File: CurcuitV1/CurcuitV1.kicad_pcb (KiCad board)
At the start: 2 copper layers, 40 x 40 mm, 46 parts, among them IC1 AS5600-ASOT, J1 Conn_01x07, J2 Conn_01x03, J3 Conn_01x02, J4 Conn_01x02, Q1 Q_NMOS_DGS, Q2 Q_NMOS_DGS, Q3 Q_NMOS_DGS, Q4 Q_NMOS_DGS, Q5 Q_NMOS_DGS, Q6 Q_NMOS_DGS, SW1 SW_Push, U1 IR2302, U2 IR2302, U3 IR2302, U4 STM32F303K8Tx, U5 LM1117MP-3.3, Y2 CSTNE16M0V530000R0

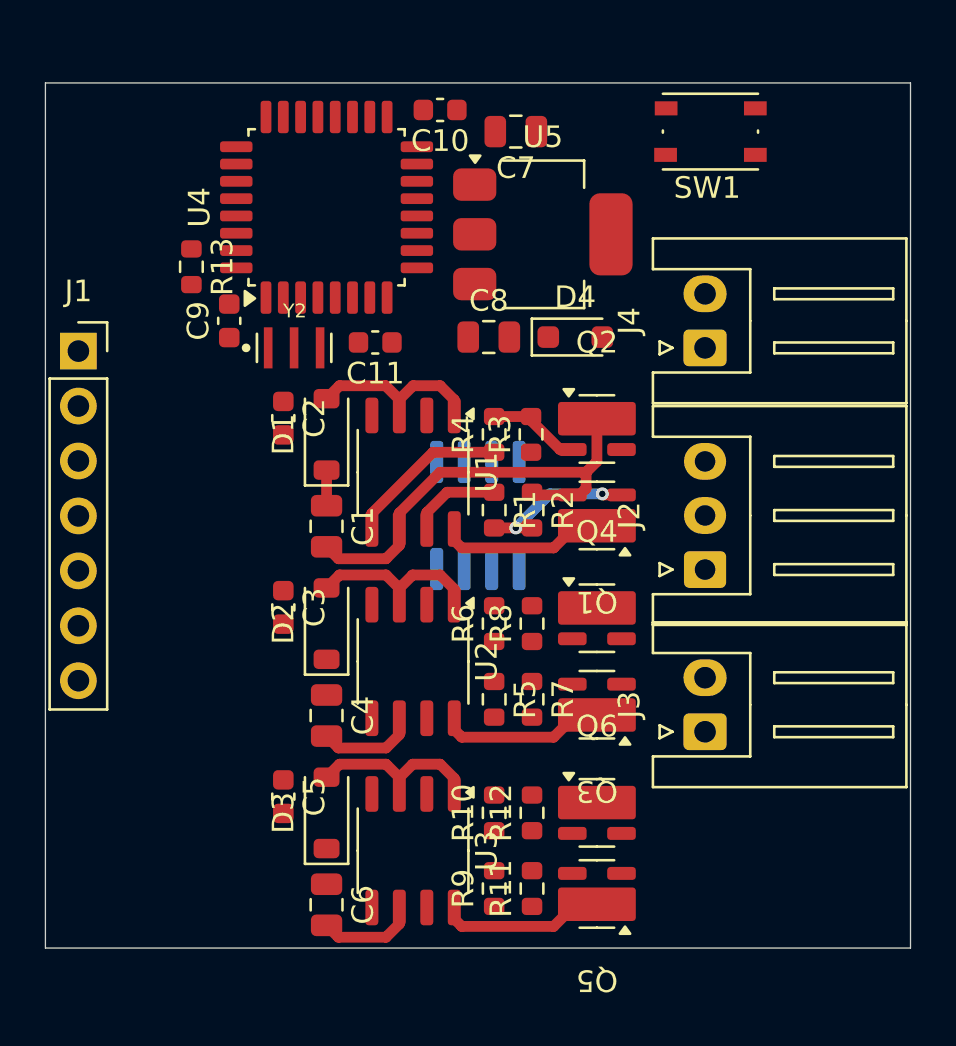
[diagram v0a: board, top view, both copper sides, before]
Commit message: 大体完成
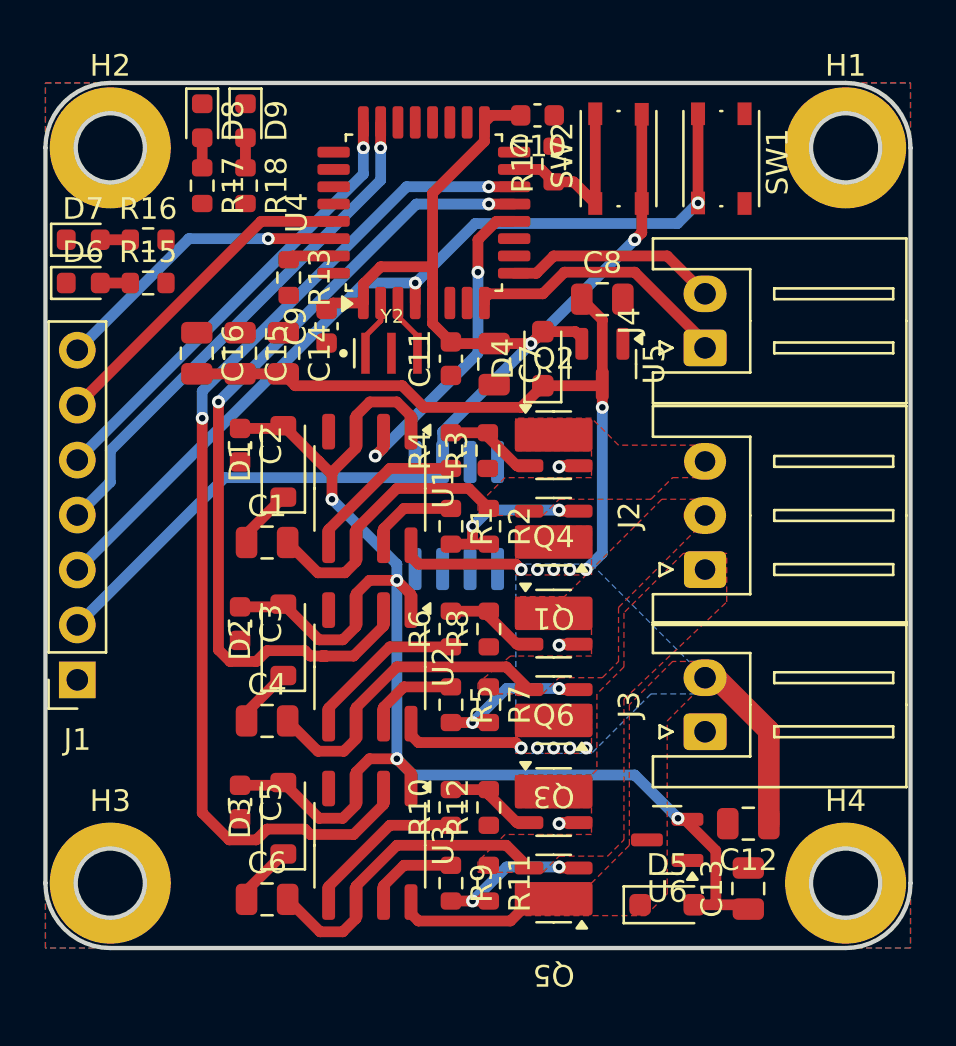
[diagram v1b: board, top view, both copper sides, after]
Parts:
- added C12: 10u, Capacitor_SMD:C_0805_2012Metric, F.Cu at (132.5, 134.2)
- added C13: 10u, Capacitor_SMD:C_0805_2012Metric, F.Cu at (132.5, 137.2)
- added C14: 10u, Capacitor_SMD:C_0805_2012Metric, F.Cu at (111.0, 112.5)
- added C15: 10u, Capacitor_SMD:C_0805_2012Metric, F.Cu at (109.0, 112.5)
- added C16: 10u, Capacitor_SMD:C_0805_2012Metric, F.Cu at (107.0, 112.5)
- added D5: D_Schottky, Diode_SMD:D_SOD-323_HandSoldering, F.Cu at (128.8, 138.0)
- added D6: LED, LED_SMD:LED_0603_1608Metric, F.Cu at (101.8, 109.2)
- added D7: LED, LED_SMD:LED_0603_1608Metric, F.Cu at (101.8, 107.2)
- added D8: LED, LED_SMD:LED_0603_1608Metric, F.Cu at (107.2, 101.8)
- added D9: LED, LED_SMD:LED_0603_1608Metric, F.Cu at (109.2, 101.8)
- added H1: MountingHole, MountingHole:MountingHole_3.2mm_M3_DIN965_Pad, F.Cu at (137.0, 103.0)
- added H2: MountingHole, MountingHole:MountingHole_3.2mm_M3_DIN965_Pad, F.Cu at (103.0, 103.0)
- added H3: MountingHole, MountingHole:MountingHole_3.2mm_M3_DIN965_Pad, F.Cu at (103.0, 137.0)
- added H4: MountingHole, MountingHole:MountingHole_3.2mm_M3_DIN965_Pad, F.Cu at (137.0, 137.0)
- added R14: 10k, Resistor_SMD:R_0603_1608Metric, F.Cu at (123.5, 103.8)
- added R15: 1k, Resistor_SMD:R_0603_1608Metric, F.Cu at (104.8, 109.2)
- added R16: 1k, Resistor_SMD:R_0603_1608Metric, F.Cu at (104.8, 107.2)
- added R17: 1k, Resistor_SMD:R_0603_1608Metric, F.Cu at (107.2, 104.8)
- added R18: 1k, Resistor_SMD:R_0603_1608Metric, F.Cu at (109.2, 104.8)
- added SW2: SW_Push, Button_Switch_SMD:SW_Push_1P1T_NO_Vertical_Wuerth_434133025816, F.Cu at (126.5, 103.5)
- added U6: AP7375-3.3, Package_TO_SOT_SMD:SOT-23, F.Cu at (128.8, 135.0)
- U5: value LM1117MP-3.3 -> AP7375-3.3; footprint Package_TO_SOT_SMD:SOT-223-3_TabPin2 -> Package_TO_SOT_SMD:SOT-23
- moved J1 15.2 mm to (101.5, 127.6), turned to 180 degrees
- moved C7 10.8 mm to (120.8, 113.0), turned to -90 degrees
- moved U5 6.60 mm to (125.8, 113.0), turned to -90 degrees
- moved C8 5.53 mm to (125.8, 110.0)
- moved R13 4.53 mm to (111.2, 109.0)
- moved C10 4.51 mm to (122.8, 101.5)
- moved C9 4.51 mm to (113.0, 111.2)
- moved U4 4.51 mm to (117.5, 106.0)
- moved Y2 4.51 mm to (116.0, 112.5)
- moved C11 3.58 mm to (118.8, 112.8), turned to 90 degrees
- moved C1 2.85 mm to (110.2, 121.2), turned to 0 degrees
- moved C4 2.76 mm to (110.2, 129.5), turned to 0 degrees
- moved C6 2.76 mm to (110.2, 137.8), turned to 0 degrees
- moved C2 2.36 mm to (109.0, 116.8)
- moved D1 2.36 mm to (111.0, 117.5)
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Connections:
- J1 pad 3: unconnected-(J1-Pin_3-Pad3) -> NSRT
- J1 pad 4: unconnected-(J1-Pin_4-Pad4) -> SWDIO
- J1 pad 5: unconnected-(J1-Pin_5-Pad5) -> SWCLK
- J1 pad 6: unconnected-(J1-Pin_6-Pad6) -> PC_TX
- J1 pad 7: unconnected-(J1-Pin_7-Pad7) -> PC_RX
- J4 pad 1: GND -> UART2_TX
- J4 pad 2: VCC -> UART2_RX
- U4 pad 12: unconnected-(U4-PA6-Pad12) -> U_IN
- U4 pad 13: unconnected-(U4-PA7-Pad13) -> V_IN
- U4 pad 14: unconnected-(U4-PB0-Pad14) -> W_IN
- U4 pad 15: unconnected-(U4-PB1-Pad15) -> BUTTON
- U4 pad 29: unconnected-(U4-PB6-Pad29) -> PC_TX
- U4 pad 30: unconnected-(U4-PB7-Pad30) -> PC_RX
- U4 pad 8: unconnected-(U4-PA2-Pad8) -> UART2_TX
- U4 pad 9: unconnected-(U4-PA3-Pad9) -> UART2_RX
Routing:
- net +3V3: track 0.00 -> 67.3 mm, vias 0 -> 2
- net W_IN: track 0.00 -> 48.4 mm, vias 0 -> 2
- net +5V: track 25.2 -> 71.5 mm, vias 0 -> 4
- net NSRT: track 0.00 -> 40.8 mm, vias 0 -> 2
- net V_IN: track 0.00 -> 38.9 mm, vias 0 -> 2
- net VCC: track 24.6 -> 63.2 mm, vias 0 -> 11
- net SWDIO: track 0.00 -> 24.0 mm, vias 0 -> 1
- net SWCLK: track 0.00 -> 21.1 mm, vias 0 -> 1
- net PC_TX: track 0.00 -> 15.4 mm
- net U_IN: track 0.00 -> 15.3 mm, vias 0 -> 2
- net PC_RX: track 0.00 -> 14.0 mm, vias 0 -> 1
- net UART2_TX: track 0.00 -> 12.5 mm
- net V_OUT: track 4.61 -> 15.4 mm
- net W_OUT: track 4.61 -> 14.8 mm
- net UART2_RX: track 0.00 -> 9.88 mm
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- added copper zone on B.Cu, net GND
- added copper zone on F.Cu, net GND
- added copper zone on F.Cu, net U_OUT
- added copper zone on B.Cu, net VCC
- added copper zone on F.Cu, net VCC
- added copper zone on F.Cu, net V_OUT
- added copper zone on F.Cu, net W_OUT
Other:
- outline, holes or cut-outs redrawn
- board text added: "+"
- board text added: "-"
- board text added: "3V3"
- board text added: "BLDC Driver V1.0 Designed by Bambi"
- board text added: "CLK"
- board text added: "DIO"
- board text added: "GND"
- board text added: "NSRT"
- board text added: "RX"
- board text added: "TX"
- board text added: "U"
- board text added: "V"
- board text added: "W"
